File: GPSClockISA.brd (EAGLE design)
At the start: 98.7 x 83.8 mm, 45 parts, among them IC1 74LS85N, IC2 74HC138N, IC3 27C512AP, IC4 74HC688N, IC5 8250/16450, IC6 74HC138N, X1 1.8432MHz, X2 53047-08

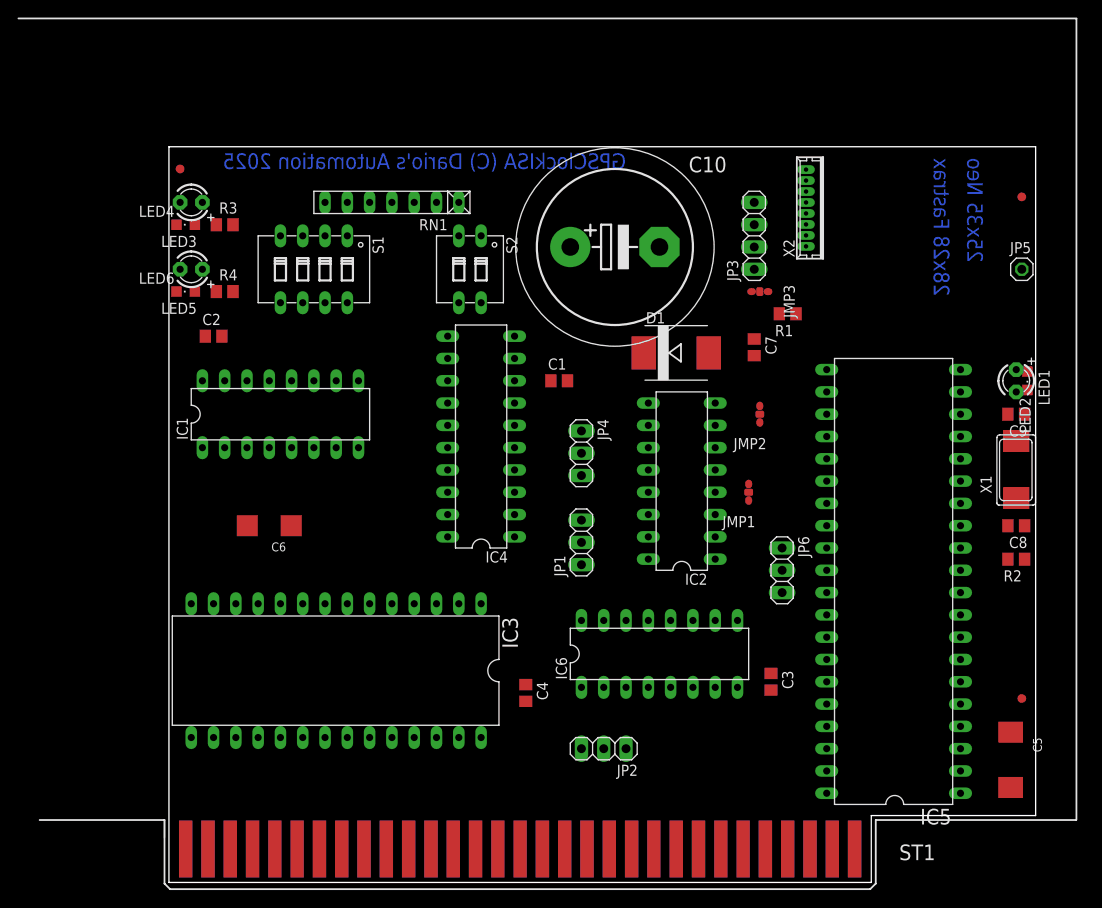
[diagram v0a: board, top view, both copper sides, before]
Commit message: Add files via upload
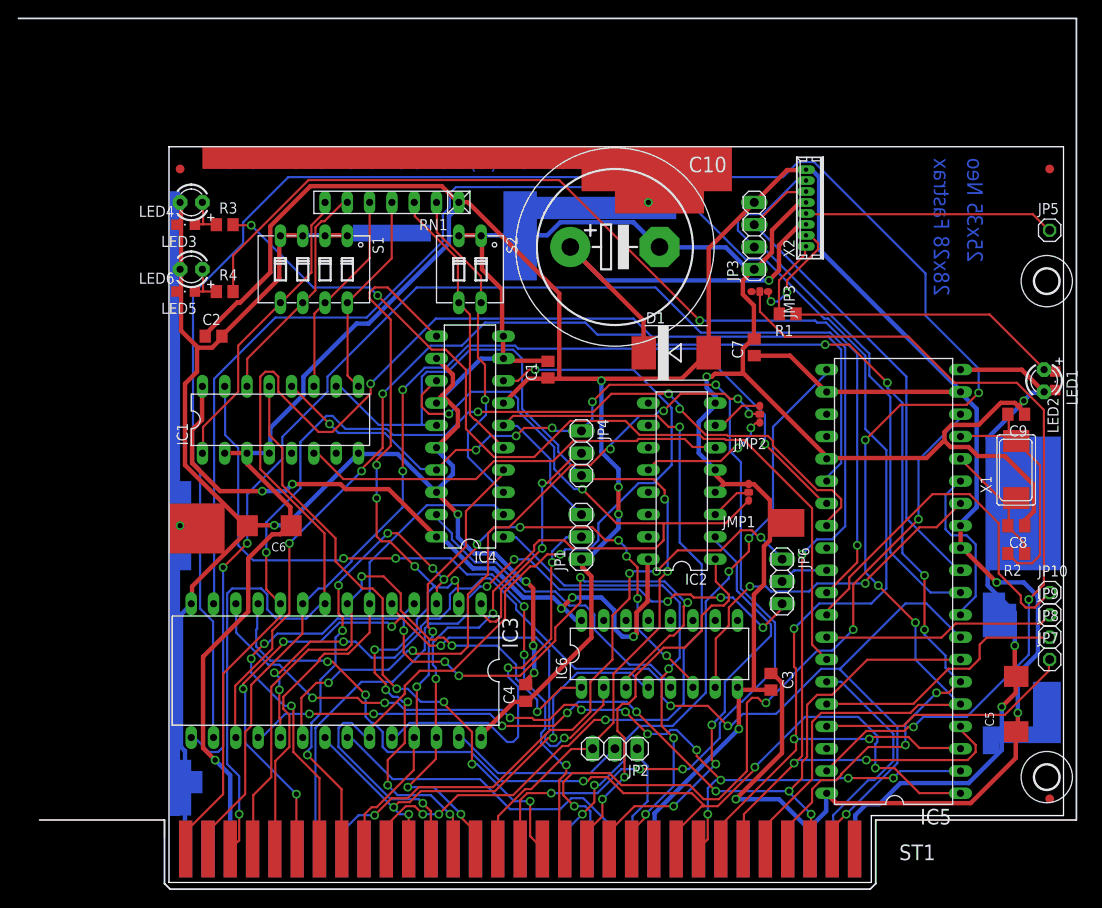
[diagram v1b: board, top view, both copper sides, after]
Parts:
- added H1, H2: MOUNT-HOLEM3, holes:M3
- added JP10, JP7, JP8, JP9: (no value), pinhead:1X01
- moved F3 11.9 mm to (100.3, 9.53)
- moved C5 6.38 mm to (96.5, 20.3), turned to 90 degrees
- moved JP5 5.46 mm to (100.3, 74.3)
- moved F1 4.49 mm to (100.3, 81.3)
- moved LED1 3.17 mm to (101.0, 57.1)
- moved LED2 3.17 mm to (99.7, 57.1)
- moved C1 1.80 mm to (43.2, 58.4), turned to 90 degrees
- moved IC4 1.27 mm to (34.3, 50.8)
- moved JP6 1.27 mm to (69.8, 34.3)
- moved JP2 1.27 mm to (50.8, 15.2)
- moved IC1 0.64 mm to (12.7, 52.7)
- moved R2 0.64 mm to (96.5, 37.5)
- moved JP1 0.63 mm to (47.0, 39.4)
- turned C4 to 90 degrees
- turned C7 to 90 degrees
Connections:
- new net N$26: IC5.37, JP7.1
- new net N$27: IC5.36, JP8.1
- new net N$28: IC5.33, JP9.1
- new net N$29: IC5.32, JP10.1
- net BA13: now also JMP1.1
- net BA15: no longer JMP1.1
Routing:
- net GND: track 0.00 -> 487.7 mm, vias 0 -> 10
- net +5V: track 0.00 -> 433.6 mm, vias 0 -> 7
- net BD4: track 0.00 -> 248.1 mm, vias 0 -> 4
- net BD2: track 0.00 -> 208.1 mm, vias 0 -> 3
- net BD3: track 0.00 -> 205.5 mm, vias 0 -> 5
- net BD5: track 0.00 -> 178.8 mm, vias 0 -> 9
- net BA2: track 0.00 -> 167.0 mm, vias 0 -> 2
- net BD7: track 0.00 -> 135.0 mm, vias 0 -> 6
- net BA15: track 0.00 -> 134.8 mm, vias 0 -> 9
- net BA0: track 0.00 -> 128.1 mm, vias 0 -> 4
- net BA1: track 0.00 -> 121.7 mm, vias 0 -> 3
- net BA13: track 0.00 -> 117.5 mm, vias 0 -> 6
- net OUT2: track 0.00 -> 115.6 mm, vias 0 -> 2
- net BD0: track 0.00 -> 112.4 mm, vias 0 -> 5
- net BA9: track 0.00 -> 112.2 mm, vias 0 -> 4
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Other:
- board size 98.7 x 83.8 mm -> 101.9 x 83.8 mm
